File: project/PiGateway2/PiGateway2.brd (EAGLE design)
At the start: 65 x 30 mm, 19 parts

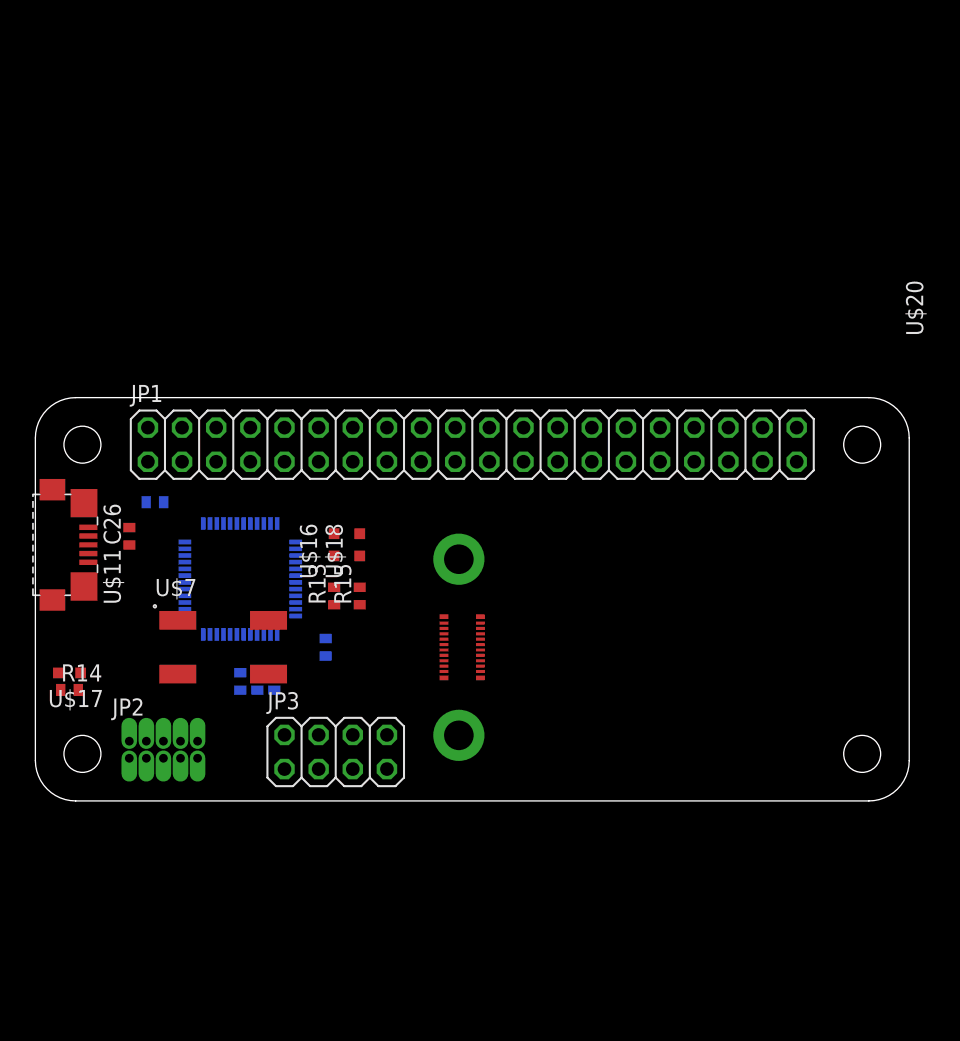
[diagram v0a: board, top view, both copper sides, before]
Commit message: fixed Pi Gateway2
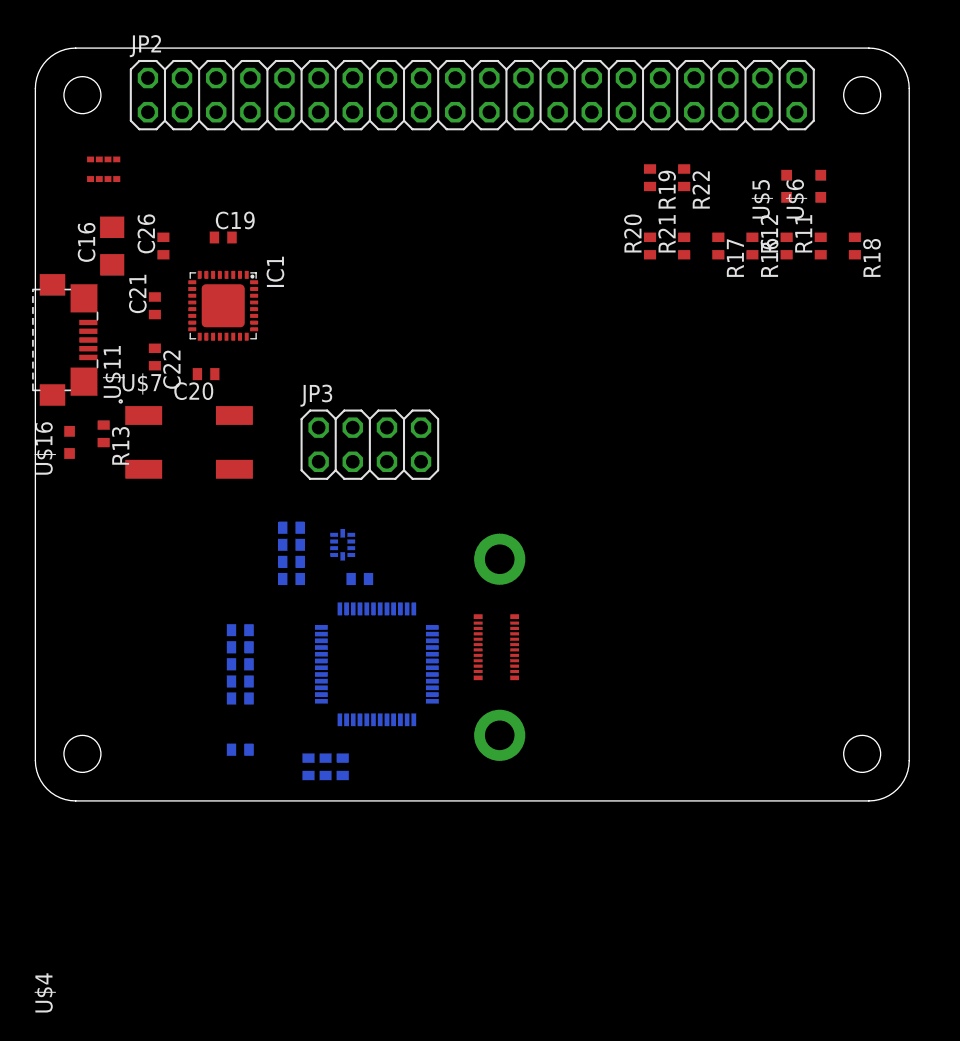
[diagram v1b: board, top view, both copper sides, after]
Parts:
- removed JP1: (no value), pinhead:2X20
- removed R14, R15: 1K, rcl:R0402
- removed U$17: SML-E12Y8W, lazurite:SML-E1X
- removed U$18: SML-E13BC8T, lazurite:SML-E1X
- removed U$20: DF40C-20DP-0.4V(51), lazurite:BP3596A
- added C16: 22u, rcl:C1206
- added C19, C20, C24: 0.1u, rcl:C0402
- added C21, C22: 47p, rcl:C0402
- added IC1: FT232RQ, ftdichip:QFN32
- added R1, R5, R6: 510, rcl:R0402
- added R10, R16, R17, R18, R19, R22, R4, R9: 10K, rcl:R0402
- added R11, R12, R7, R8: 1K, rcl:R0402
- added R20: 0, rcl:R0402
- added R21: NC, rcl:R0402
- added U$2: RT1A060AP, lz-shield:TSST8
- added U$3: TI-TS5A23159, lz-shield:UQFN10
- added U$4: DF40C-20DP-0.4V(51), lazurite:BP3596A
- added U$5: SML-E13BC8T, lazurite:SML-E1X
- added U$6: SML-E12Y8W, lazurite:SML-E1X
- JP2: value PINHD_2X5_HALF -> (none); device lazurite:PINHD_2X5_HALF -> pinhead:2X20
- moved JP2 52.2 mm to (32.5, 52.5)
- moved JP3 23.0 mm to (24.9, 26.5)
- moved C26 21.7 mm to (9.53, 41.3)
- moved U$16 21.1 mm to (2.54, 26.7)
- moved R13 21.0 mm to (5.08, 27.3), turned to 270 degrees
- moved U$7 15.5 mm to (11.4, 26.7)
- moved U$11 15.2 mm to (1.27, 34.3)
- moved U$1 12.0 mm to (25.4, 10.2)
- moved C1 11.7 mm to (19.1, 16.5)
- moved C3 8.13 mm to (20.3, 2.54)
- moved C4 8.13 mm to (21.6, 2.54)
- moved C5 8.13 mm to (22.9, 2.54), turned to 90 degrees
- moved C2 6.48 mm to (15.2, 12.7), turned to 180 degrees
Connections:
- removed net 3V: U$20.8, U$20.9
- removed net MISO0: U$20.12
- removed net MISO0I: U$1.20
- removed net MOSI0: U$20.16
- removed net MOSI0I: U$1.19
- removed net N$22: JP1.35
- removed net N$23: JP1.37
- removed net N$24: JP1.40
- removed net N$25: JP1.38
- removed net N$26: JP1.36
- removed net N$27: JP1.32
- removed net N$31: JP1.22
- removed net N$32: JP1.18
- removed net N$33: JP1.16
- removed net N$35: JP1.10
- removed net NFC_IRQI: U$1.38
- removed net RF_CSBI: U$1.2
- removed net RF_IRQI: U$1.32
- removed net RF_REGPDINI: U$1.37
- removed net RF_RSTBI: U$1.3
- removed net SCL0: U$20.1
- removed net SCL0I: U$1.26
- removed net SCLK0: U$20.14
- removed net SCLK0I: U$1.21
- removed net SDA0: U$20.2
- removed net SDA0I: U$1.25
- new net +5V/1: C1.1, C16.1, C19.1, C2.1, C20.1, C24.1, C26.1, C5.1, IC1.1, IC1.19, JP3.1, R10.1, R13.2, R9.1, U$1.12, U$1.13, U$1.44, U$11.1, U$2.P5, U$3.8
- new net BOOT_WRITE: IC1.11, R4.1, U$3.1, U$3.5
- new net DM: C22.1, IC1.15, U$11.2
- new net DP: C21.1, IC1.14, U$11.3
- new net I2C_SCL: JP2.5, R17.2, U$4.1
- new net I2C_SDA: JP2.3, R16.2, U$4.2
- new net LED_RX: JP2.33, U$6.C
- new net LED_TX: JP2.31, U$5.C
- new net M2P: JP2.7
- new net MISO: JP2.21, U$4.12
- new net MOSI: JP2.19, U$4.16
- new net N$1: JP2.15
- new net N$2: R1.2
- new net N$37: R11.2, U$6.A
- new net N$38: R12.2, U$5.A
- new net P2M: JP2.8
- new net RF_CSB0: JP2.24, R19.2, R20.2
- new net RF_CSB1: JP2.26, R21.2, R22.2
- new net SCLK: JP2.23, U$4.14
- new net U_TEST0: R6.1, U$3.9
- new net U_TEST1N: R5.1, U$3.7
- net +3V3: now also JP2.1, JP2.17, R11.1, R12.1, R16.1, R17.1, R18.1, R19.1, R22.1, U$4.8, U$4.9; no longer JP1.1, JP1.17, R14.1, R15.1
- net +5V: now also JP2.2, U$2.P1, U$2.P2, U$2.P3, U$2.P6, U$2.P8; no longer C1.1, C2.1, C26.1, C5.1, JP1.2, JP1.4, JP2.0, JP2.1, JP2.5, R13.2, U$1.12, U$1.13, U$1.44, U$11.1
- net AVDD_MON: now also U$4.7; no longer U$20.7
- net EEP_WP: now also U$4.18; no longer U$20.18
- net GND: now also C16.2, C19.2, C20.2, C21.2, C22.2, C24.2, IC1.17, IC1.20, IC1.24, IC1.26, IC1.4, JP2.14, JP2.20, JP2.25, JP2.30, JP2.34, JP2.39, JP2.6, JP2.9, JP3.8, R4.2, U$3.3, U$4.17, U$4.3, U$4.4, U$4.5, U$4.6, U$4.GND1; no longer JP1.14, JP1.20, JP1.25, JP1.30, JP1.34, JP1.39, JP1.6, JP1.9, JP2.2, JP2.3, U$20.17, U$20.3, U$20.4, U$20.5, U$20.6, U$20.GND1
- net N$10: now also JP2.29; no longer JP1.5
- net N$11: now also JP2.35; no longer JP1.7
- net N$12: now also JP2.37; no longer JP1.11
- net N$13: now also JP2.40; no longer JP1.13
- net N$14: now also IC1.2, R8.2; no longer JP1.15
- net N$15: now also JP2.38; no longer JP1.19
- net N$16: now also JP2.36; no longer JP1.21
- net N$17: now also JP2.32; no longer JP1.23
- net N$18: now also IC1.22, R6.2; no longer JP1.27
- net N$19: now also IC1.21, R5.2; no longer JP1.29
- net N$20: now also JP2.28; no longer JP1.31
- net N$21: now also JP2.22; no longer JP1.33
- net N$28: now also R1.1, U$2.P4; no longer JP1.28
- net N$29: now also JP2.18; no longer JP1.26
- net N$30: now also JP2.16; no longer JP1.24
- net N$34: now also JP2.10; no longer JP1.8
- net N$36: now also U$4.GND2; no longer JP1.12
- net N$4: now also IC1.32, U$3.2; no longer U$20.GND2
- net N$5: now also IC1.31, U$3.4; no longer R14.2, U$17.A
- net N$6: now also IC1.30, R7.2; no longer R15.2, U$18.A
- net N$9: now also JP2.27; no longer JP1.3
- net P30: now also R7.1
- net P31: now also R8.1
- net P34: now also JP3.5, R9.2
- net P35: now also JP3.6, R10.2
- net P36: now also JP3.4
- net P44: now also JP3.2
- net P45: now also JP3.3
- net P50: now also U$7.1, U$7.2
- net P51: no longer U$17.C
- net P53: now also JP3.7
- net P56: no longer U$18.C
- net RESETN: no longer U$7.1, U$7.2
- net RF_CSB: now also R20.1, R21.1, U$4.15; no longer U$20.15
- net RF_IRQ: now also JP2.12, U$4.13; no longer U$20.13
- net RF_REGPDIN: now also JP2.11, U$4.10; no longer U$20.10
- net RF_RSTB: now also JP2.13, R18.2, U$4.11; no longer U$20.11
- net TEST0: now also U$3.10
- net TEST1N: now also U$3.6
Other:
- board size 65 x 30 mm -> 65 x 56 mm
- board text added: "Bootが書き込めない RPi電源ON/USB oFFが考慮されていない"
